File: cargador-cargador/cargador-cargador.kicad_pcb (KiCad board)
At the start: 2 copper layers, 15 x 20 mm, 7 parts, among them J1 Jack DC, J2 salida, U1 L7805

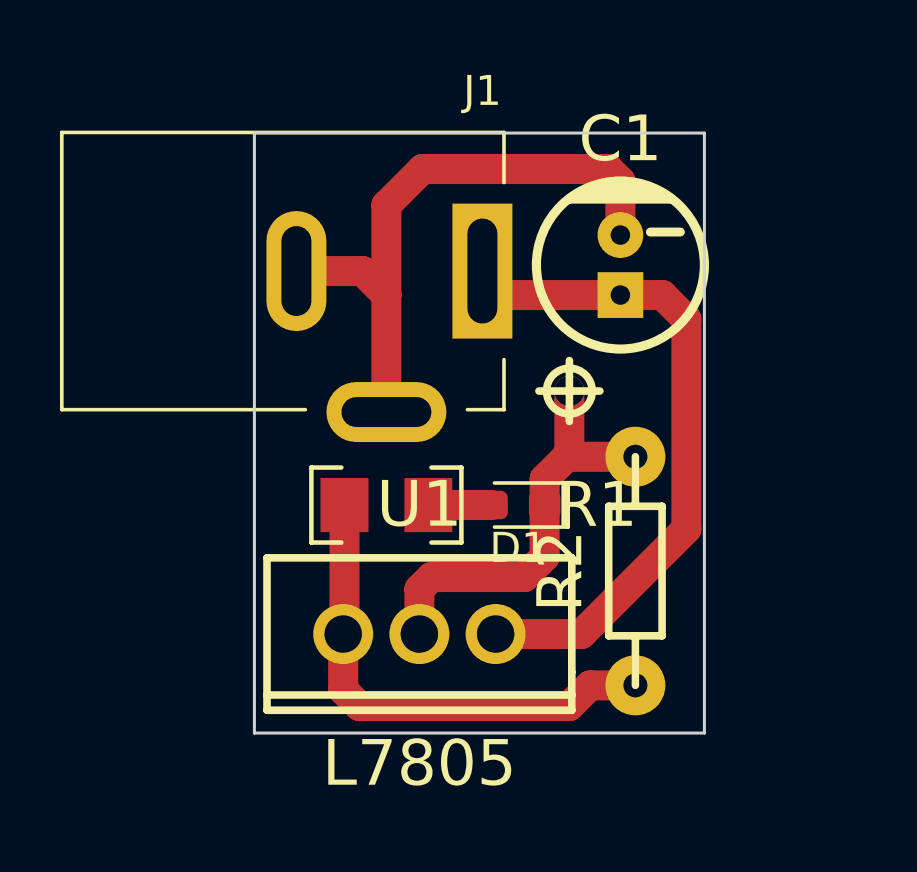
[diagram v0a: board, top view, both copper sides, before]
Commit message: little responsive
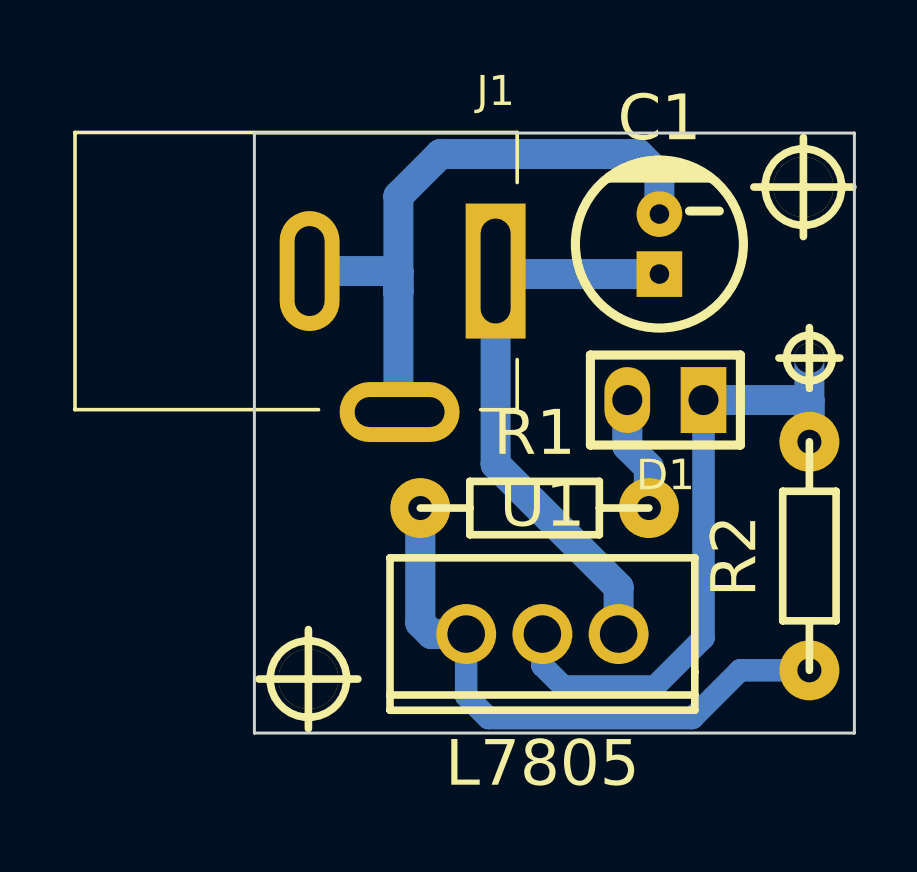
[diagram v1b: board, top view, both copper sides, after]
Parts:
- added hole_2mm: VAL**, EESTN5:hole_2mm, F.Cu at (78.3, 41.8)
- added hole_2mm: VAL**, EESTN5:hole_2mm, F.Cu at (61.8, 58.2)
- D1: footprint LED_SMD:LED_0603_1608Metric_Pad1.05x0.95mm_HandSolder -> EESTN5:Pin_strip_2
- R1: footprint EESTN5:R_1206 -> EESTN5:RES0.3
- moved J2 8.08 mm to (78.5, 47.5)
- moved D1 6.02 mm to (73.7, 48.9)
- moved R2 5.82 mm to (78.5, 54.1)
- moved R1 4.94 mm to (69.3, 52.5), turned to 0 degrees
- moved U1 4.10 mm to (69.6, 56.7)
- moved C1 1.48 mm to (73.5, 43.7)
- moved J1 0.44 mm to (68.0, 44.6)
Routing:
- net Net-(D1-K): track 14.3 -> 23.0 mm
- net Net-(U1-OUT): track 16.4 -> 20.0 mm
- net Net-(U1-IN): track 22.3 -> 19.3 mm
- net Net-(D1-A): track 2.13 -> 3.90 mm
- net GND: track 20.5 -> 21.7 mm
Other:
- board size 15 x 20 mm -> 20 x 20 mm
